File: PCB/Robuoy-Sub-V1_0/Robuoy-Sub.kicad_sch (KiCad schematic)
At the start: 6 parts

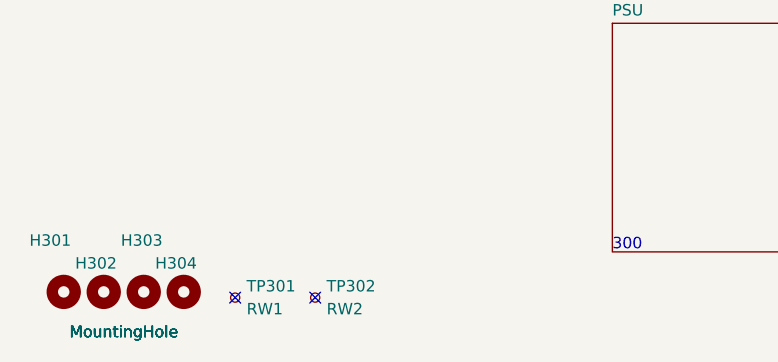
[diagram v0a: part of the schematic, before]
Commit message: Pcb edditing
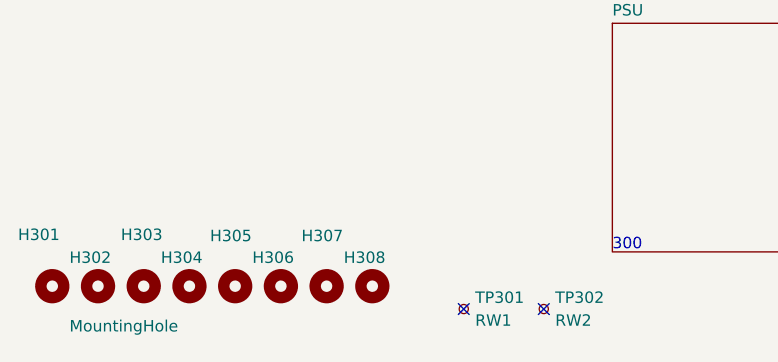
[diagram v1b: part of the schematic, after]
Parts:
- added H305, H306, H307, H308: MountingHole, A_Mechanical:NPTH_M3, symbol Mechanical:MountingHole
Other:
- moved on the sheet: H301, H302, H303, H304, TP301, TP302
